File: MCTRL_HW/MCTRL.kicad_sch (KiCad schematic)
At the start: 22 parts, among them Q1 NMOS, Q2 NMOS, Q3 NMOS, Q4 NMOS, U1 IR2110, U2 IR2110

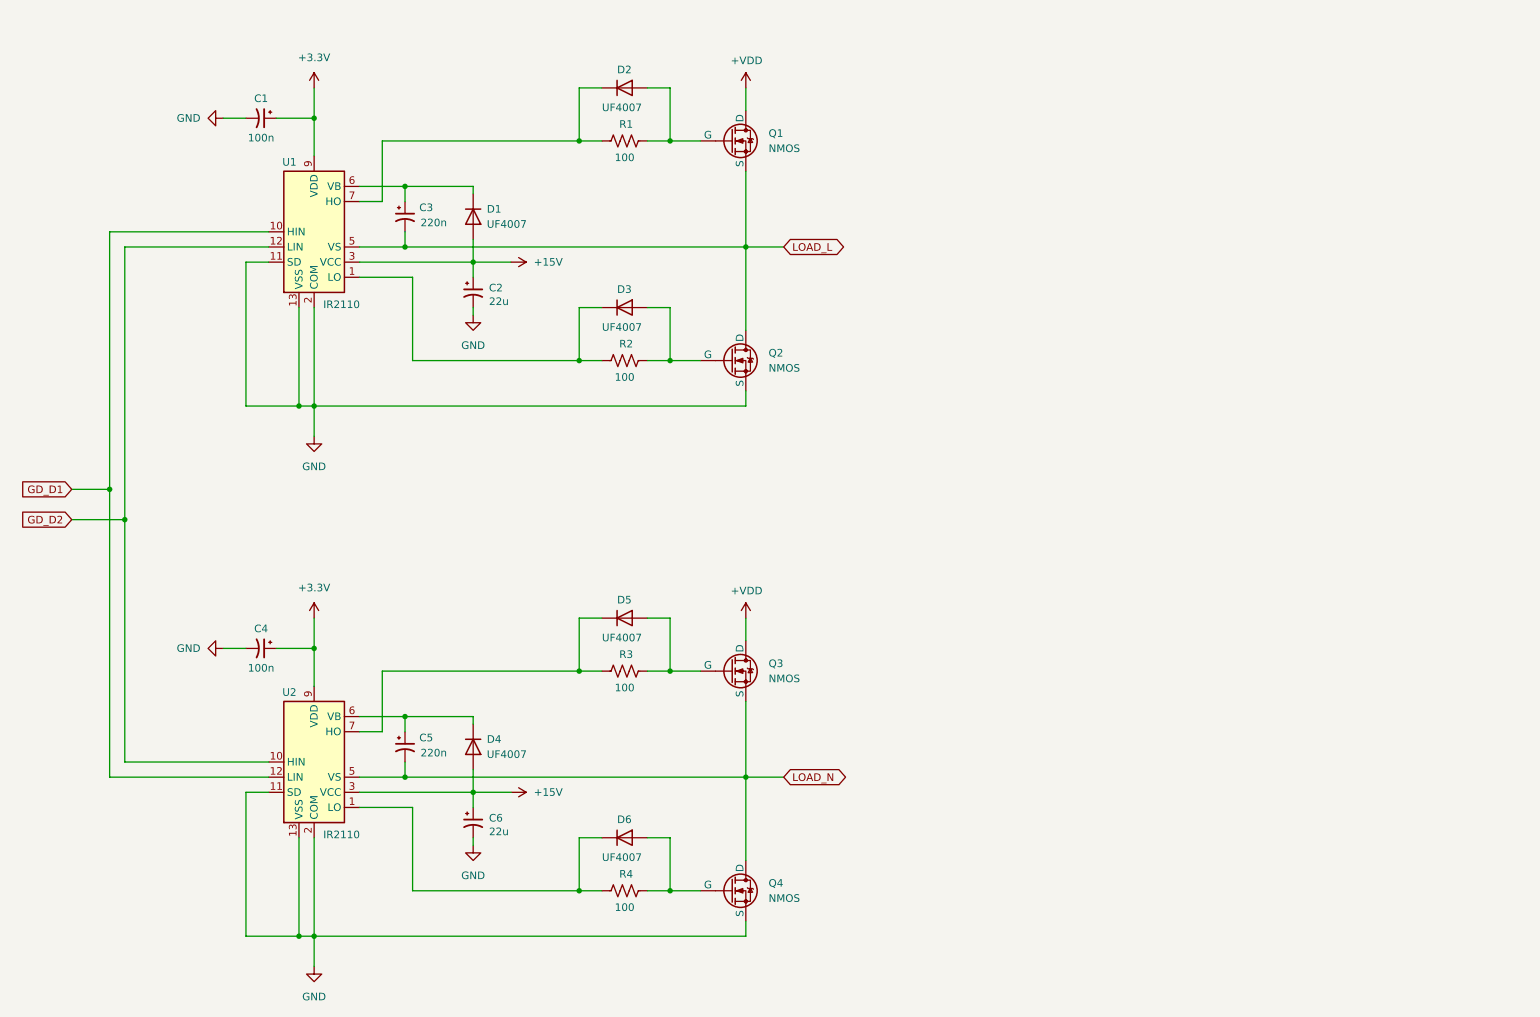
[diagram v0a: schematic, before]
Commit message: more changes
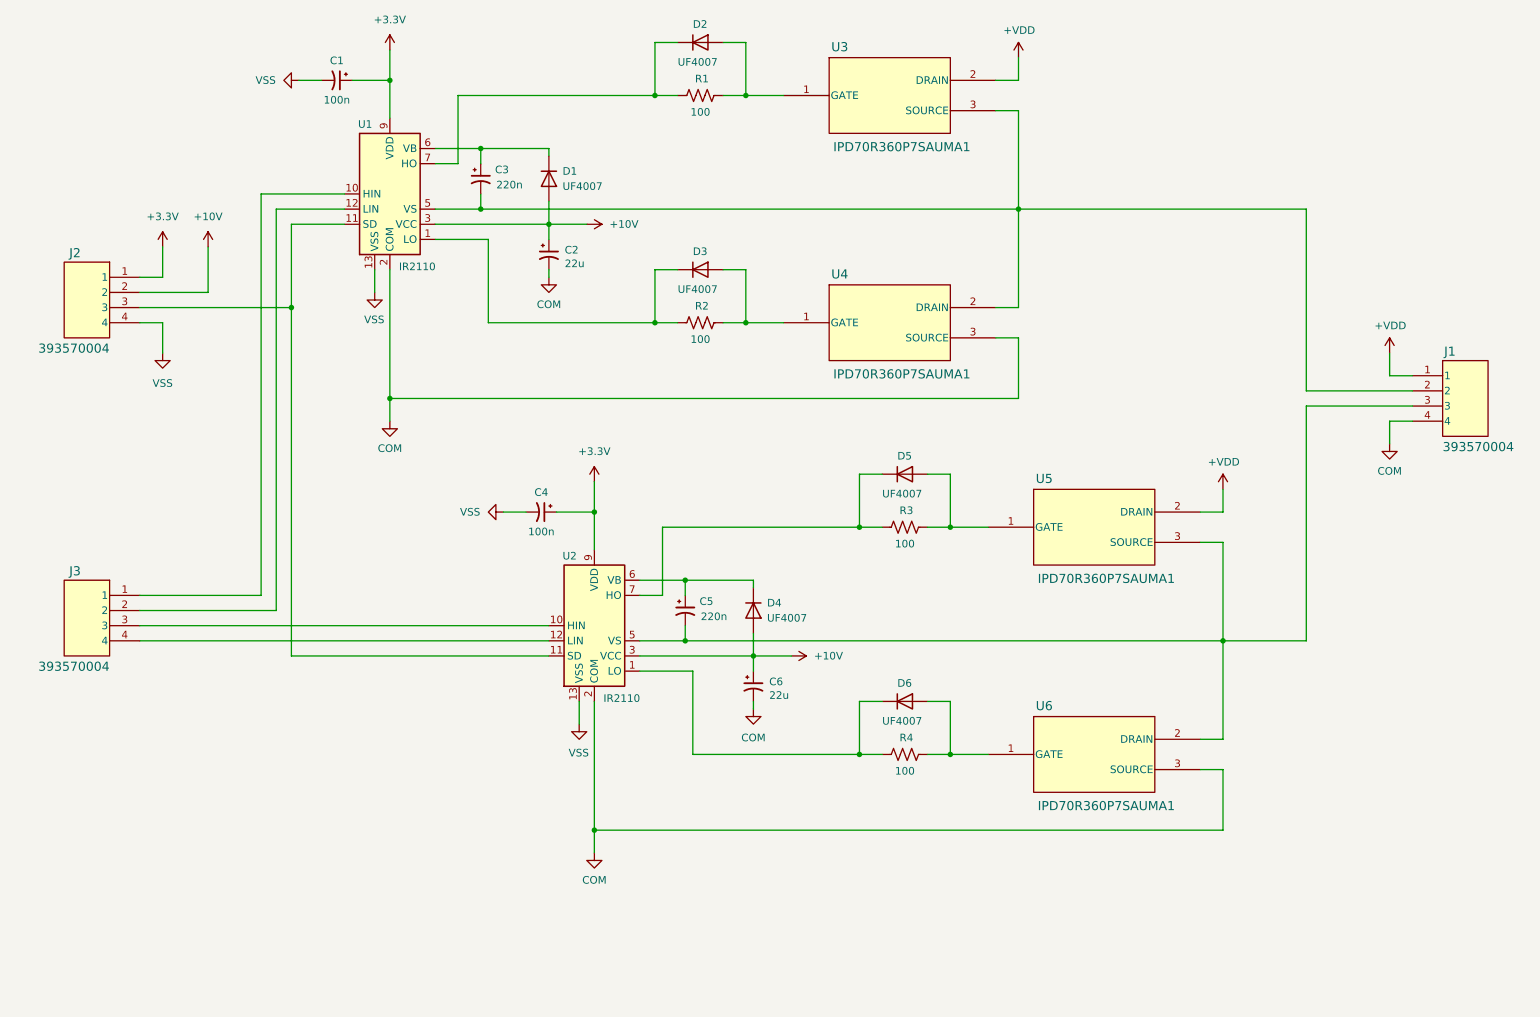
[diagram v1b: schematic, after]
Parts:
- removed Q1, Q2, Q3, Q4: NMOS, symbol Simulation_SPICE:NMOS
- added J1, J2, J3: 393570004, MCTRL:393570004, symbol MCTRL:393570004
- added U3, U4, U5, U6: IPD70R360P7SAUMA1, MCTRL:IPD70R360P7SAUMA1, symbol MCTRL:IPD70R360P7SAUMA1
- D1, D4: footprint (none) -> Diode_THT:D_DO-15_P12.70mm_Horizontal
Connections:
- net +3.3V: now also J2.1
- net +VDD: now also J1.1, U3.2 (DRAIN), U5.2 (DRAIN)
- net at D6.2 (A), R4.2: now also U6.1 (GATE)
- net at D2.2 (A), R1.2: now also U3.1 (GATE)
- net at D3.2 (A), R2.2: now also U4.1 (GATE)
- net at D5.2 (A), R3.2: now also U5.1 (GATE)
- net +15V renamed +10V
- net +10V: now also J2.2
- net GD_D1: no longer names the net of U1.10 (HIN)
- net GD_D1: now also J3.1; no longer U2.12 (LIN)
- net GD_D2: no longer names the net of U1.12 (LIN)
- net GD_D2: now also J3.2; no longer U2.10 (HIN)
- removed net GND: C1.2, C2.2, C4.2, C6.2, U1.11 (SD), U1.13 (VSS), U1.2 (COM), U2.11 (SD), U2.13 (VSS), U2.2 (COM)
- net LOAD_L: no longer names the net of C3.2, U1.5 (VS)
- net LOAD_L: now also J1.2, U3.3 (SOURCE), U4.2 (DRAIN)
- net LOAD_N: no longer names the net of C5.2, U2.5 (VS)
- net LOAD_N: now also J1.3, U5.3 (SOURCE), U6.2 (DRAIN)
- new net: J3.3, U2.10 (HIN)
- new net: J3.4, U2.12 (LIN)
- new net: J2.3, U1.11 (SD), U2.11 (SD)
- new net COM: C2.2, C6.2, J1.4, U1.2 (COM), U2.2 (COM), U4.3 (SOURCE), U6.3 (SOURCE)
- new net VSS: C1.2, C4.2, J2.4, U1.13 (VSS), U2.13 (VSS)
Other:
- moved on the sheet: C1, C2, C3, C4, C5, C6, D1, D2, D3, D4, D5, D6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
